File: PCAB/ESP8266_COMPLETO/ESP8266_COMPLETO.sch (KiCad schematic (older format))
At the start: 2 parts, among them J1 USB_B_Micro, U1 ESP32-WROOM-32

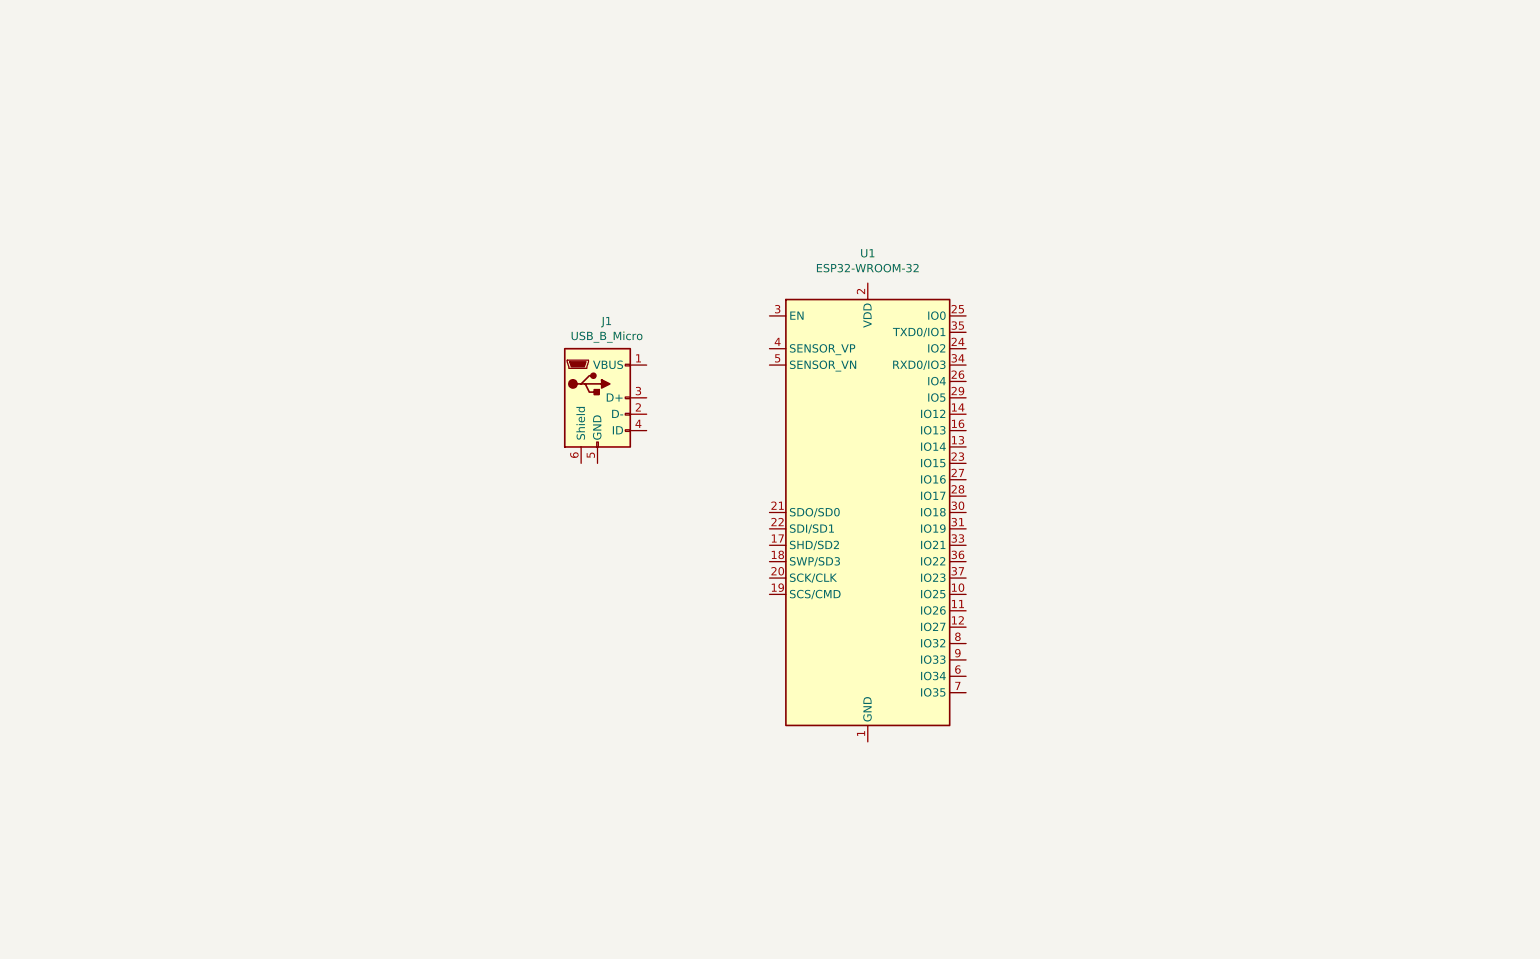
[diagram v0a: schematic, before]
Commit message: PCB relays completa
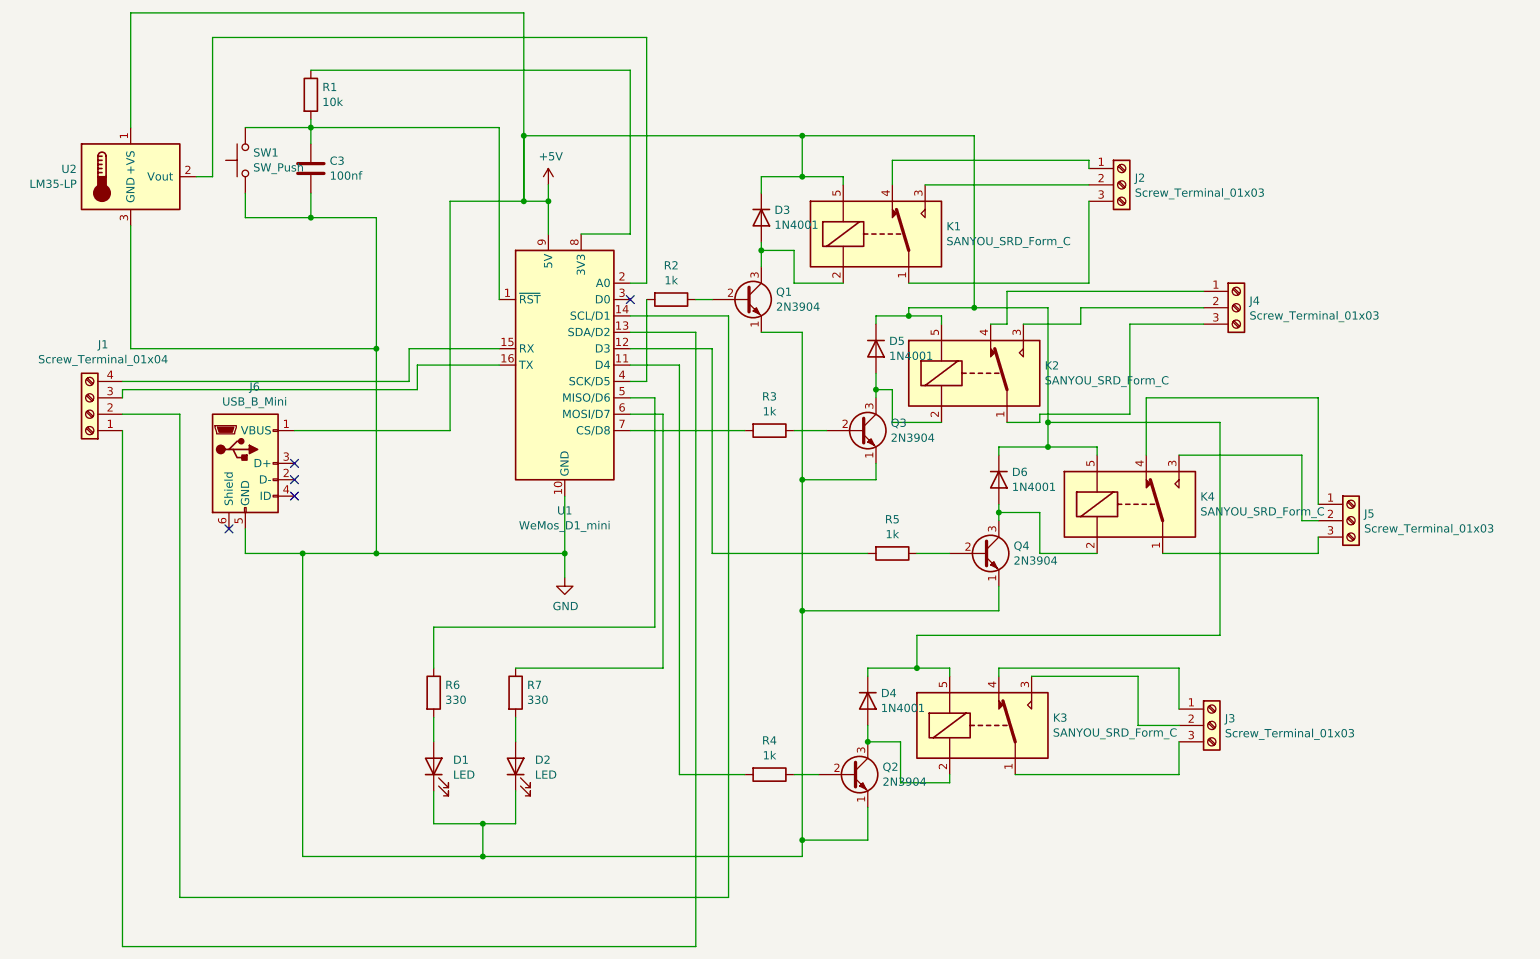
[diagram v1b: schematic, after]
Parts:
- removed J1: USB_B_Micro, Connector_USB:USB_Micro-AB_Molex_47590-0001, symbol Connector:USB_B_Micro
- removed U1: ESP32-WROOM-32, RF_Module:ESP32-WROOM-32, symbol RF_Module:ESP32-WROOM-32
- added C3: 100nf, Capacitor_THT:C_Disc_D5.0mm_W2.5mm_P5.00mm, symbol Device:C
- added D1, D2: LED, LED_THT:LED_D5.0mm, symbol Device:LED
- added D3, D4, D5, D6: 1N4001, Diode_THT:D_DO-41_SOD81_P10.16mm_Horizontal, symbol Diode:1N4001
- added J1: Screw_Terminal_01x04, Connector:FanPinHeader_1x04_P2.54mm_Vertical, symbol Connector:Screw_Terminal_01x04
- added J2, J3, J4, J5: Screw_Terminal_01x03, TerminalBlock_Phoenix:TerminalBlock_Phoenix_MKDS-1,5-3-5.08_1x03_P5.08mm_Horizontal, symbol Connector:Screw_Terminal_01x03
- added J6: USB_B_Mini, Connector_USB:USB_Mini-B_Lumberg_2486_01_Horizontal, symbol Connector:USB_B_Mini
- added K1, K2, K3, K4: SANYOU_SRD_Form_C, Relay_THT:Relay_SPDT_SANYOU_SRD_Series_Form_C, symbol Relay:SANYOU_SRD_Form_C
- added Q1, Q2, Q3, Q4: 2N3904, Package_TO_SOT_THT:TO-92_Inline, symbol Transistor_BJT:2N3904
- added R1: 10k, Resistor_THT:R_Axial_DIN0204_L3.6mm_D1.6mm_P7.62mm_Horizontal, symbol Device:R
- added R2, R3, R4, R5: 1k, Resistor_THT:R_Axial_DIN0204_L3.6mm_D1.6mm_P7.62mm_Horizontal, symbol Device:R
- added R6, R7: 330, Resistor_THT:R_Axial_DIN0204_L3.6mm_D1.6mm_P7.62mm_Horizontal, symbol Device:R
- added SW1: SW_Push, Button_Switch_THT:SW_PUSH_6mm, symbol Switch:SW_Push
- added U1: WeMos_D1_mini, Module:WEMOS_D1_mini_light, symbol MCU_Module:WeMos_D1_mini
- added U2: LM35-LP, Package_TO_SOT_THT:TO-92_Inline, symbol Sensor_Temperature:LM35-LP
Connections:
- new net: C3.1, R1.2, SW1.2, U1.1 (~RST)
- new net: R4.2, U1.11 (D4)
- new net: R5.2, U1.12 (D3)
- new net: J1.1 (Pin_1), U1.13 (SDA/D2)
- new net: J1.2 (Pin_2), U1.14 (SCL/D1)
- new net: J1.4 (Pin_4), U1.15 (RX)
- new net: J1.3 (Pin_3), U1.16 (TX)
- new net: U1.2 (A0), U2.2 (Vout)
- new net: R2.2, U1.4 (SCK/D5)
- new net: R6.1, U1.5 (MISO/D6)
- new net: R7.1, U1.6 (MOSI/D7)
- new net: R3.2, U1.7 (CS/D8)
- new net: R1.1, U1.8 (3V3)
- new net: Q1.2 (B), R2.1
- new net: D3.2 (A), K1.2, Q1.3 (C)
- new net: Q2.2 (B), R4.1
- new net: D4.2 (A), K3.2, Q2.3 (C)
- new net: Q4.2 (B), R5.1
- new net: D6.2 (A), K4.2, Q4.3 (C)
- new net: Q3.2 (B), R3.1
- new net: D5.2 (A), K2.2, Q3.3 (C)
- new net: J2.1 (Pin_1), K1.4
- new net: J2.2 (Pin_2), K1.3
- new net: J2.3 (Pin_3), K1.1
- new net: J4.1 (Pin_1), K2.4
- new net: J4.2 (Pin_2), K2.3
- new net: J4.3 (Pin_3), K2.1
- new net: J5.1 (Pin_1), K4.4
- new net: J5.2 (Pin_2), K4.3
- new net: J5.3 (Pin_3), K4.1
- new net: J3.1 (Pin_1), K3.4
- new net: J3.2 (Pin_2), K3.3
- new net: J3.3 (Pin_3), K3.1
- new net: D1.2 (A), R6.2
- new net: D2.2 (A), R7.2
- new net +5V: D3.1 (K), D4.1 (K), D5.1 (K), D6.1 (K), J6.1 (VBUS), K1.5, K2.5, K3.5, K4.5, U1.9 (5V), U2.1 (+VS)
- new net GND: C3.2, D1.1 (K), D2.1 (K), J6.5 (GND), Q1.1 (E), Q2.1 (E), Q3.1 (E), Q4.1 (E), SW1.1, U1.10 (GND), U2.3 (GND)
- no-connect marks 0 -> 5
